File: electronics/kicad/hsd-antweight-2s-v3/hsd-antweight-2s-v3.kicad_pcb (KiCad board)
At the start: 2 copper layers, 78 x 56 mm, 10 parts, among them J10 3V3 GND VLIPO, J4 BATTERY, J5 MOTOR LEFT, J6 MOTOR RIGHT, SW1 SW EXT VBAT_RAW/VBAT_SW, U1 ESP32-C3 SUPERMINI, U2 DRV8833, U3 EXT REG LOGIC VIN GND VOUT

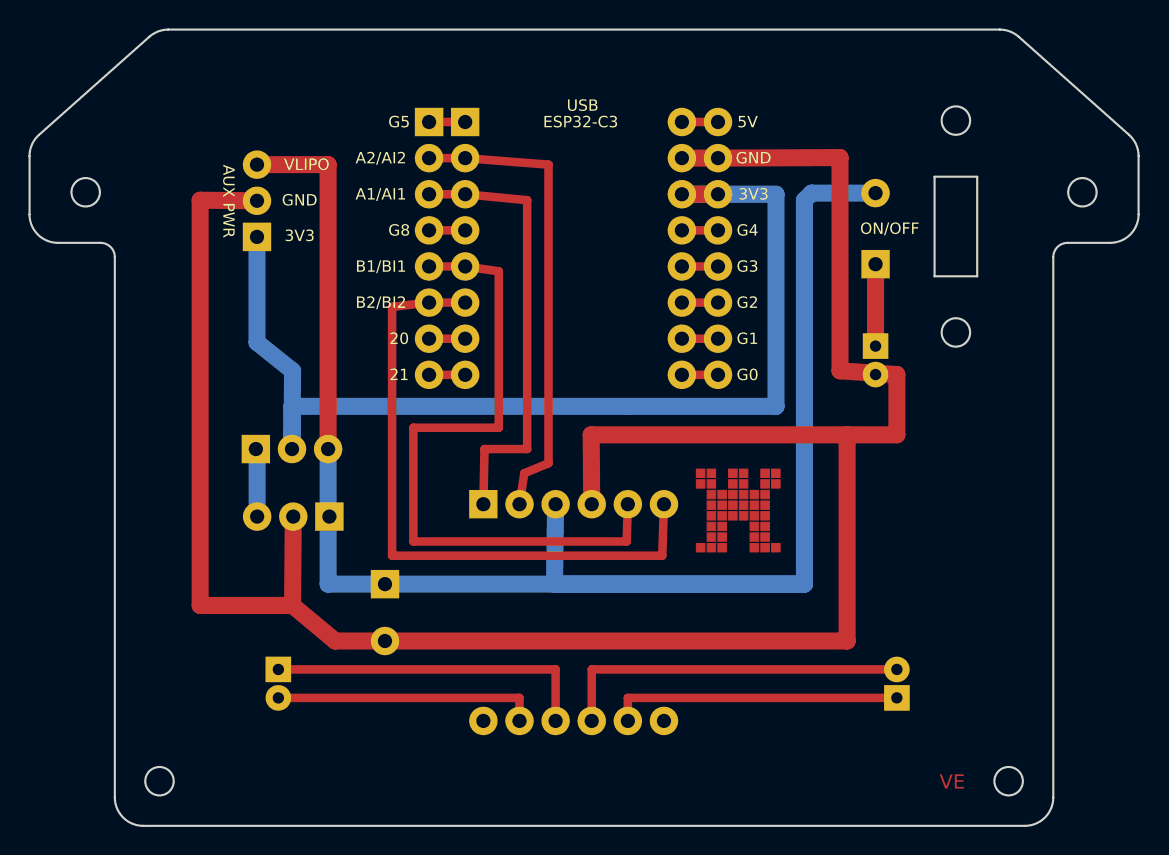
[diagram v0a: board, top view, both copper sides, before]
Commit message: kicad v3: save latest pcb update
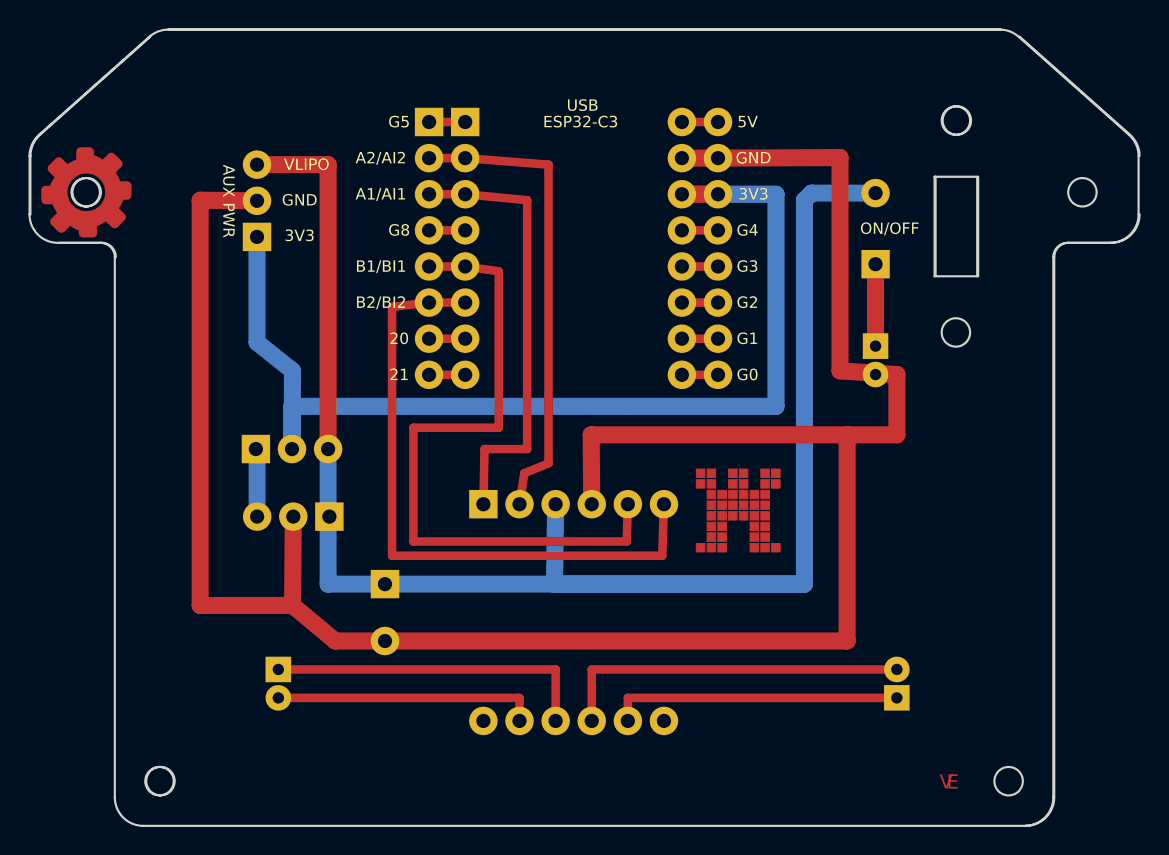
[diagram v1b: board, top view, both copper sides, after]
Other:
- board size 78 x 56 mm -> 78.1 x 56 mm
- board text added: "E"
- board text added: "V"
- board text removed: "VE"
